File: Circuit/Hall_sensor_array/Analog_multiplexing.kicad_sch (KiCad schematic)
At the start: 34 parts, among them U257 CD74HC4067SM, U258 CD74HC4067SM, U259 CD74HC4067SM, U260 CD74HC4067SM, U261 CD74HC4067SM, U262 CD74HC4067SM, U263 CD74HC4067SM, U264 CD74HC4067SM, U265 CD74HC4067SM, U266 CD74HC4067SM, U267 CD74HC4067SM, U268 CD74HC4067SM, U269 CD74HC4067SM, U270 CD74HC4067SM, U271 CD74HC4067SM, U272 CD74HC4067SM, U276 CD74HC4067SM

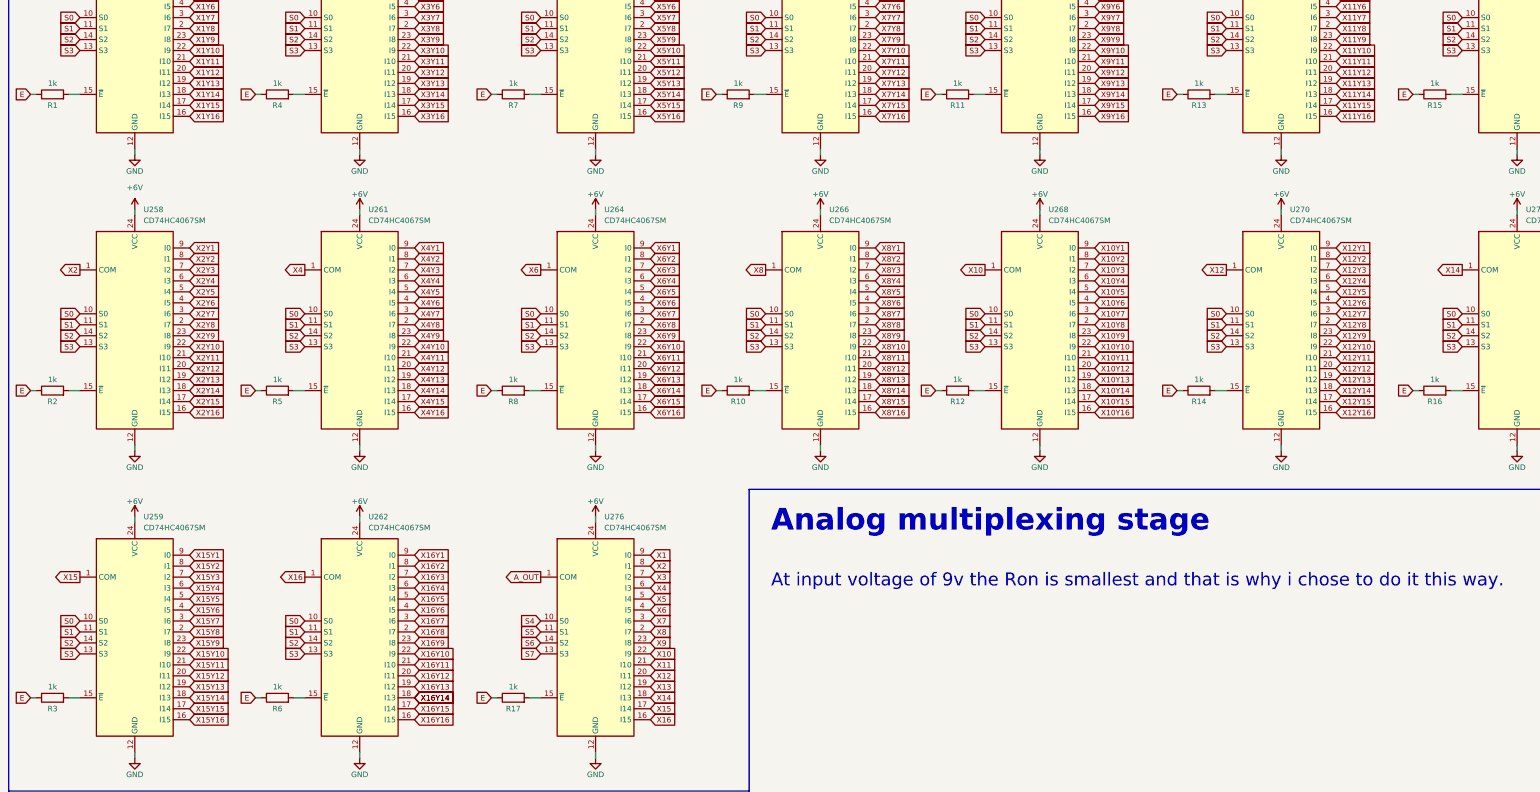
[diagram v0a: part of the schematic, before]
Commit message: Major update! New pcb
i did some work
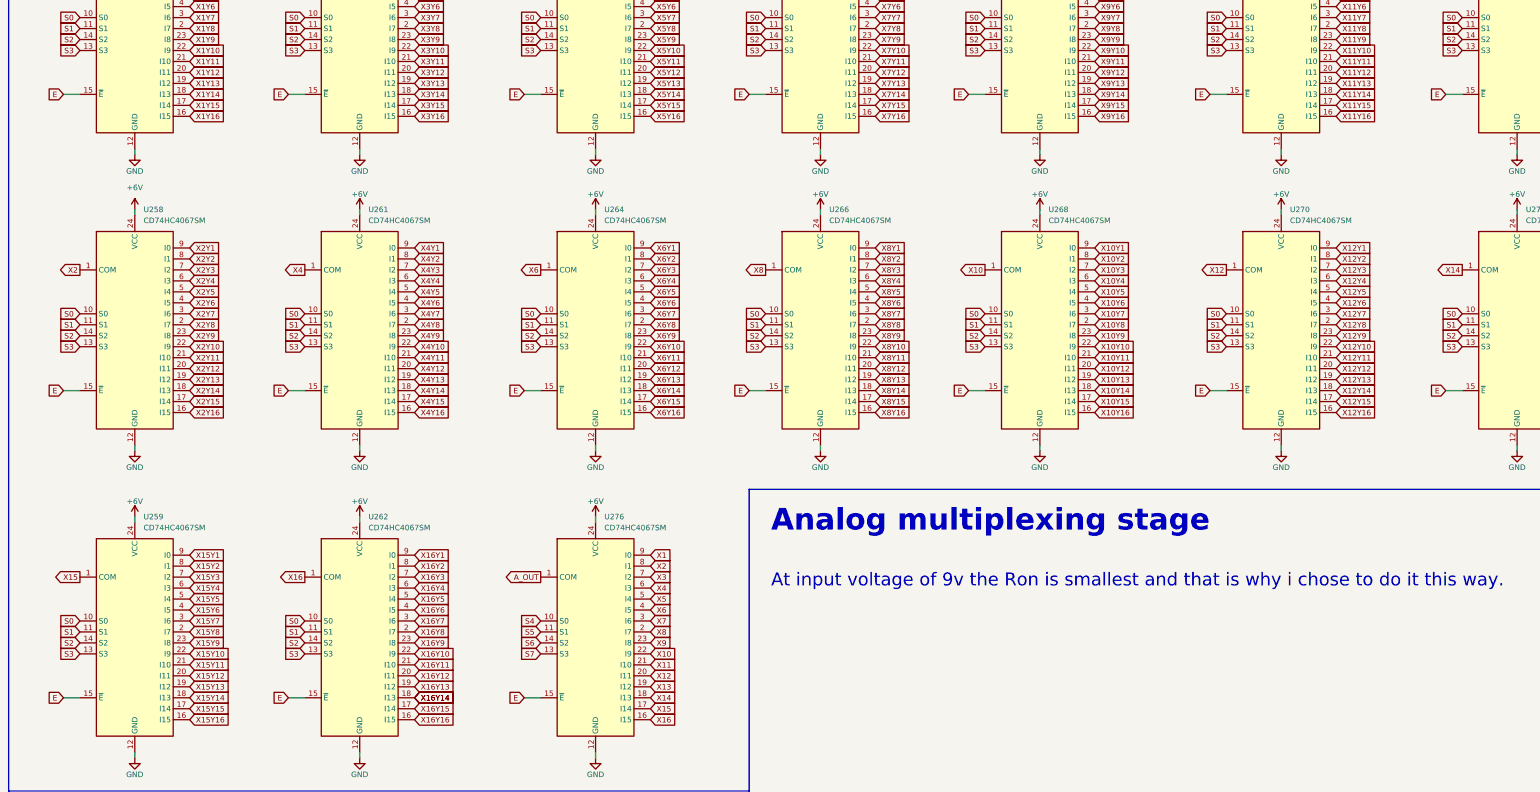
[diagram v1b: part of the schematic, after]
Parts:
- removed R1, R10, R11, R12, R13, R14, R15, R16, R17, R2, R3, R4, R5, R6, R7, R8, R9: 1k, Resistor_SMD:R_0805_2012Metric, symbol Device:R
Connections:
- net E: now also U257.15 (~{E}), U258.15 (~{E}), U259.15 (~{E}), U260.15 (~{E}), U261.15 (~{E}), U262.15 (~{E}), U263.15 (~{E}), U264.15 (~{E}), U265.15 (~{E}), U266.15 (~{E}), U267.15 (~{E}), U268.15 (~{E}), U269.15 (~{E}), U270.15 (~{E}), U271.15 (~{E}), U272.15 (~{E}), U276.15 (~{E})
